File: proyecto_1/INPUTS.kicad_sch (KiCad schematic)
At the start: 0 parts

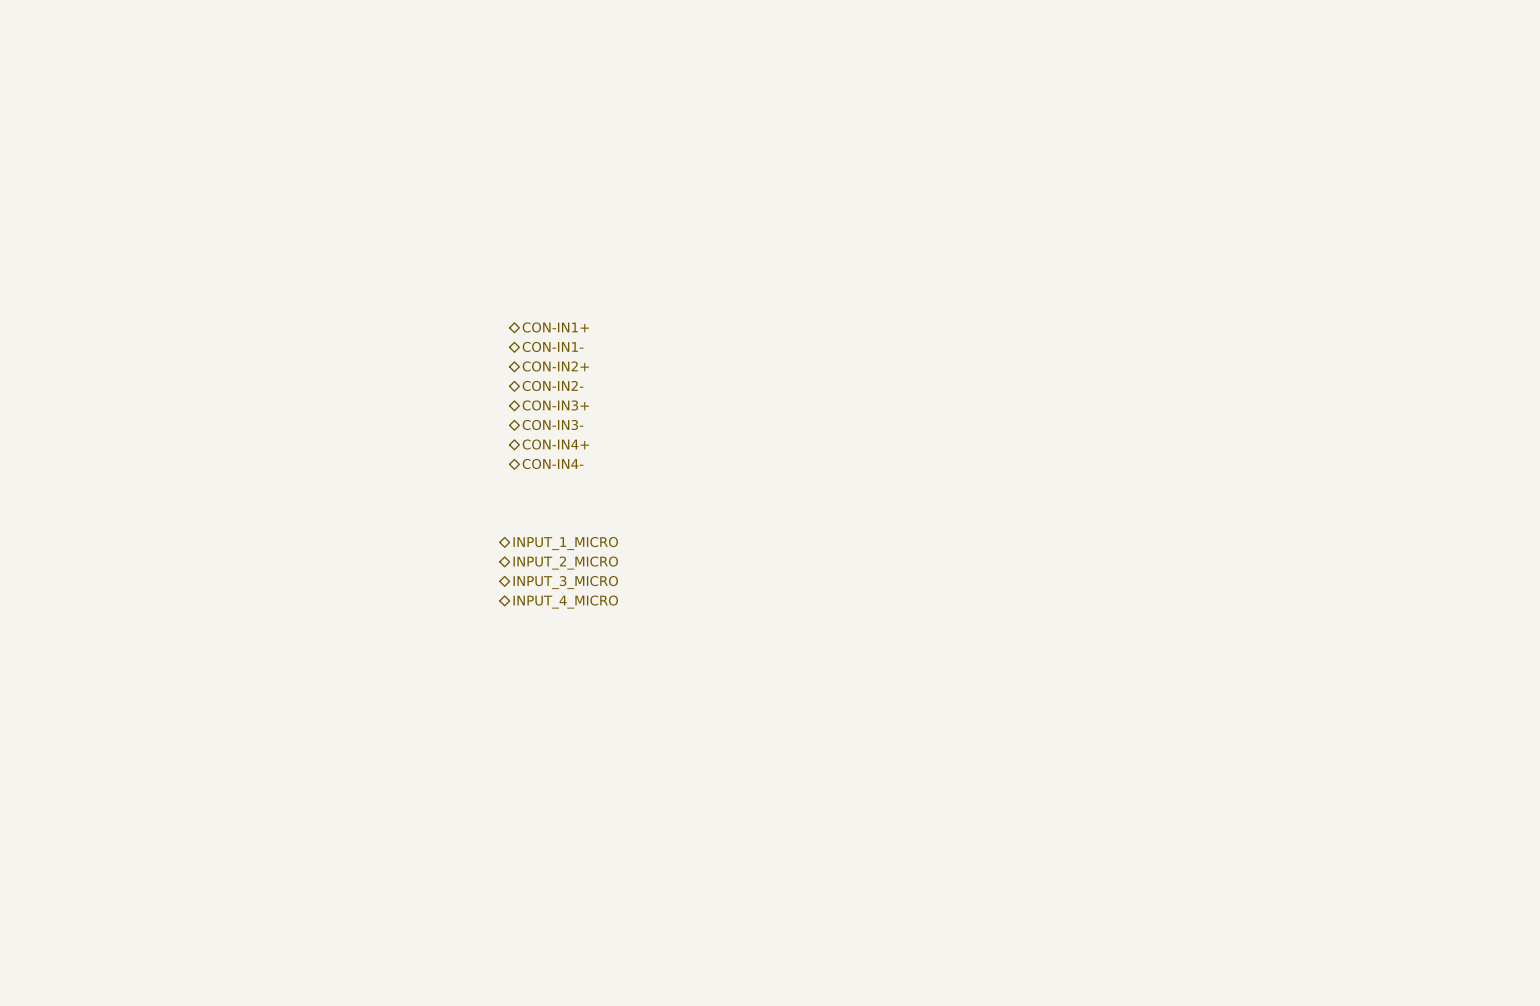
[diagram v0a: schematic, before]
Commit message: nuevos circuitos de pcb
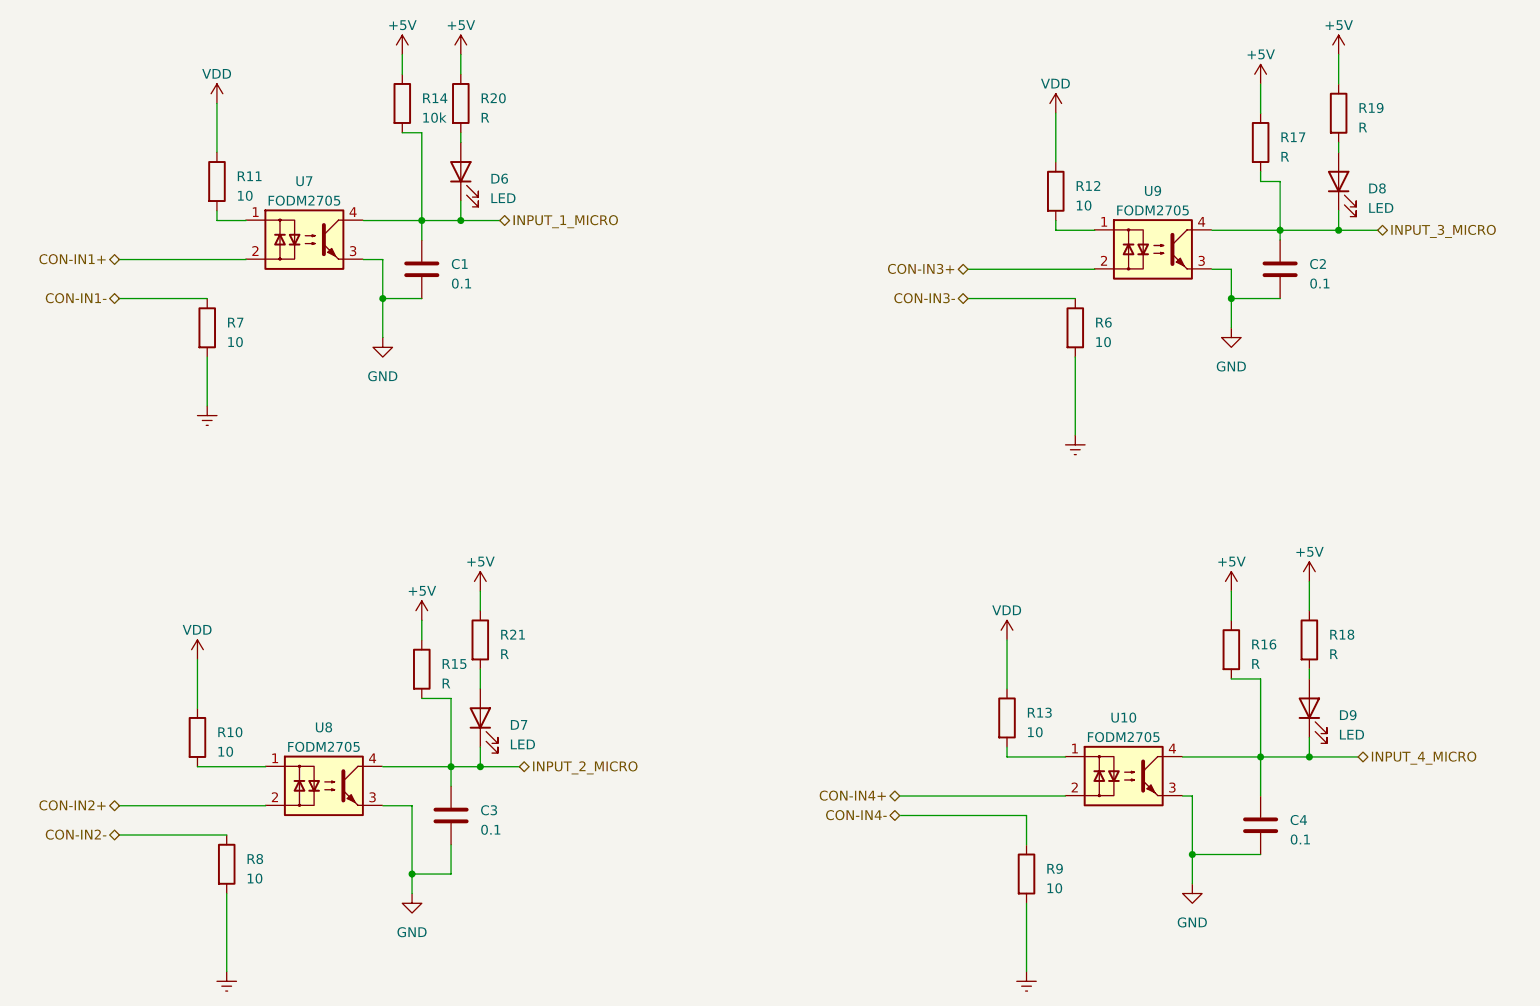
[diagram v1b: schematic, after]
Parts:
- added C1, C2, C3, C4: 0.1, symbol Device:C
- added D6, D7, D8, D9: LED, symbol Device:LED
- added R10, R11, R12, R13, R6, R7, R8, R9: 10, symbol Device:R
- added R14: 10k, symbol Device:R
- added R15, R16, R17, R18, R19, R20, R21: R, symbol Device:R
- added U10, U7, U8, U9: FODM2705, nuevo simbolo:FODM2705, symbol nuevo simbolos:FODM2705
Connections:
- net CON-IN1-: now also R7.1
- net CON-IN2-: now also R8.1
- net CON-IN3-: now also R6.1
- net CON-IN4-: now also R9.1
- net INPUT_1_MICRO: now also C1.1, D6.1 (K), R14.2
- net INPUT_2_MICRO: now also C3.1, D7.1 (K), R15.2
- net INPUT_3_MICRO: now also C2.1, D8.1 (K), R17.2
- net INPUT_4_MICRO: now also C4.1, D9.1 (K), R16.2
- new net: D8.2 (A), R19.2
- new net: D9.2 (A), R18.2
- new net: D6.2 (A), R20.2
- new net: D7.2 (A), R21.2
- new net +5V: R14.1, R15.1, R16.1, R17.1, R18.1, R19.1, R20.1, R21.1
- new net Earth: R6.2, R7.2, R8.2, R9.2
- new net GND: C1.2, C2.2, C3.2, C4.2
- new net VDD: R10.1, R11.1, R12.1, R13.1

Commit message: agregados al esquematico
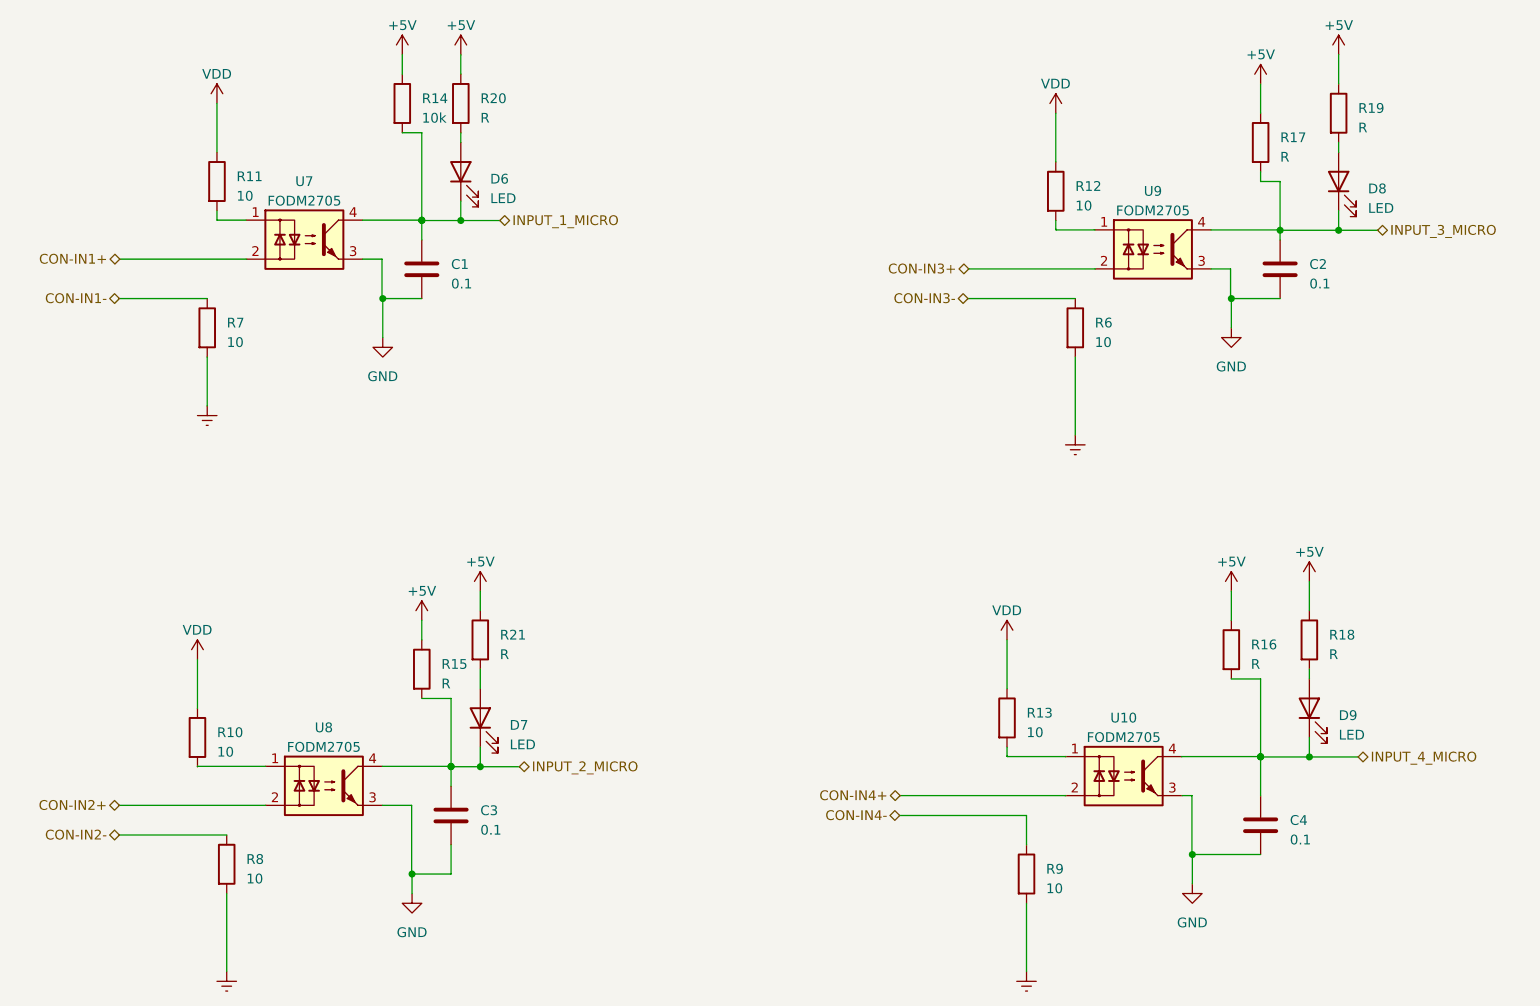
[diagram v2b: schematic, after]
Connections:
- net GND: now also U10.3, U8.3
- net INPUT_2_MICRO: now also U8.4
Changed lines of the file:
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@@
   (junction (at 214.63 64.77) (diameter 0) (color 0 0 0 0)
   )
+  (junction (at 99.06 134.5692) (diameter 0) (color 0 0 0 0)
+  )
   (junction (at 102.87 134.62) (diameter 0) (color 0 0 0 0)
   )
@@
   (junction (at 100.33 63.5) (diameter 0) (color 0 0 0 0)
   )
+  (junction (at 204.47 133.2992) (diameter 0) (color 0 0 0 0)
+  )
   (junction (at 95.25 63.5) (diameter 0) (color 0 0 0 0)
   )
@@
   (junction (at 99.06 134.62) (diameter 0) (color 0 0 0 0)
   )
+  (junction (at 95.25 63.4492) (diameter 0) (color 0 0 0 0)
+  )
   (junction (at 207.01 64.77) (diameter 0) (color 0 0 0 0)
   )
-  (wire (pts (xy 177.8 64.77) (xy 177.8 63.5))
+  (wire (pts (xy 171.45 133.2484) (xy 171.45 132.08))
+    (stroke (width 0) (type default))
+  )
+  (wire (pts (xy 177.8508 64.7192) (xy 177.8508 64.6684))
     (stroke (width 0) (type default))
   )
@@
     (stroke (width 0) (type default))
   )
+  (wire (pts (xy 90.1192 134.5692) (xy 99.06 134.5692))
+    (stroke (width 0) (type default))
+  )
   (wire (pts (xy 100.33 60.96) (xy 100.33 63.5))
     (stroke (width 0) (type default))
@@
     (stroke (width 0) (type default))
   )
-  (wire (pts (xy 179.07 133.35) (xy 171.45 133.35))
+  (wire (pts (xy 195.5292 146.05) (xy 195.58 146.05))
+    (stroke (width 0) (type default))
+  )
+  (wire (pts (xy 66.04 134.5692) (xy 66.04 134.62))
+    (stroke (width 0) (type default))
+  )
+  (wire (pts (xy 177.8 64.6684) (xy 177.8 63.5))
     (stroke (width 0) (type default))
   )
@@
     (stroke (width 0) (type default))
   )
+  (wire (pts (xy 206.9084 64.77) (xy 207.01 64.77))
+    (stroke (width 0) (type default))
+  )
+  (wire (pts (xy 90.0684 73.66) (xy 90.17 73.66))
+    (stroke (width 0) (type default))
+  )
   (wire (pts (xy 95.25 125.73) (xy 99.06 125.73))
     (stroke (width 0) (type default))
   )
-  (wire (pts (xy 72.39 63.5) (xy 68.58 63.5))
+  (wire (pts (xy 68.58 63.4492) (xy 72.39 63.4492))
     (stroke (width 0) (type default))
   )
@@
     (stroke (width 0) (type default))
   )
-  (wire (pts (xy 200.66 69.85) (xy 200.66 73.66))
+  (wire (pts (xy 200.5584 69.7992) (xy 200.5584 73.66))
     (stroke (width 0) (type default))
   )
@@
     (stroke (width 0) (type default))
   )
+  (wire (pts (xy 198.0184 69.7992) (xy 200.5584 69.7992))
+    (stroke (width 0) (type default))
+  )
   (wire (pts (xy 210.82 130.81) (xy 210.82 133.35))
     (stroke (width 0) (type default))
@@
     (stroke (width 0) (type default))
   )
+  (wire (pts (xy 99.06 134.5692) (xy 99.06 134.62))
+    (stroke (width 0) (type default))
+  )
   (wire (pts (xy 69.85 151.13) (xy 69.85 161.29))
     (stroke (width 0) (type default))
@@
     (stroke (width 0) (type default))
   )
+  (wire (pts (xy 204.47 133.2992) (xy 204.47 133.35))
+    (stroke (width 0) (type default))
+  )
   (wire (pts (xy 55.88 143.51) (xy 69.85 143.51))
     (stroke (width 0) (type default))
@@
     (stroke (width 0) (type default))
   )
-  (wire (pts (xy 194.31 133.35) (xy 204.47 133.35))
-    (stroke (width 0) (type default))
-  )
-  (wire (pts (xy 55.88 68.58) (xy 72.39 68.58))
-    (stroke (width 0) (type default))
-  )
-  (wire (pts (xy 93.98 139.7) (xy 93.98 148.59))
-    (stroke (width 0) (type default))
-  )
-  (wire (pts (xy 204.47 123.19) (xy 204.47 133.35))
-    (stroke (width 0) (type default))
-  )
-  (wire (pts (xy 66.04 134.62) (xy 74.93 134.62))
+  (wire (pts (xy 194.1576 133.2992) (xy 204.47 133.2992))
+    (stroke (width 0) (type default))
+  )
+  (wire (pts (xy 93.9292 139.6492) (xy 93.9292 148.59))
+    (stroke (width 0) (type default))
+  )
+  (wire (pts (xy 204.47 123.19) (xy 204.47 133.2992))
+    (stroke (width 0) (type default))
+  )
+  (wire (pts (xy 66.04 134.5692) (xy 74.93 134.5692))
     (stroke (width 0) (type default))
   )
@@
     (stroke (width 0) (type default))
   )
-  (wire (pts (xy 87.63 63.5) (xy 95.25 63.5))
-    (stroke (width 0) (type default))
-  )
-  (wire (pts (xy 194.31 138.43) (xy 195.58 138.43))
+  (wire (pts (xy 171.5008 133.2992) (xy 179.1208 133.2992))
+    (stroke (width 0) (type default))
+  )
+  (wire (pts (xy 95.25 63.4492) (xy 95.25 63.5))
+    (stroke (width 0) (type default))
+  )
+  (wire (pts (xy 194.2592 138.3792) (xy 195.5292 138.3792))
     (stroke (width 0) (type default))
   )
@@
     (stroke (width 0) (type default))
   )
-  (wire (pts (xy 95.25 52.07) (xy 95.25 63.5))
+  (wire (pts (xy 95.25 52.07) (xy 95.25 63.4492))
     (stroke (width 0) (type default))
   )
@@
     (stroke (width 0) (type default))
   )
-  (wire (pts (xy 166.37 69.85) (xy 182.88 69.85))
-    (stroke (width 0) (type default))
-  )
   (wire (pts (xy 195.58 146.05) (xy 204.47 146.05))
     (stroke (width 0) (type default))
   )
+  (wire (pts (xy 93.9292 148.59) (xy 93.98 148.59))
+    (stroke (width 0) (type default))
+  )
+  (wire (pts (xy 87.5284 63.4492) (xy 95.25 63.4492))
+    (stroke (width 0) (type default))
+  )
   (wire (pts (xy 204.47 45.72) (xy 204.47 49.53))
     (stroke (width 0) (type default))
   )
-  (wire (pts (xy 198.12 69.85) (xy 200.66 69.85))
-    (stroke (width 0) (type default))
-  )
-  (wire (pts (xy 157.48 138.43) (xy 179.07 138.43))
-    (stroke (width 0) (type default))
-  )
   (wire (pts (xy 214.63 53.34) (xy 214.63 54.61))
     (stroke (width 0) (type default))
   )
-  (wire (pts (xy 87.63 68.58) (xy 90.17 68.58))
+  (wire (pts (xy 200.5584 73.66) (xy 200.66 73.66))
+    (stroke (width 0) (type default))
+  )
+  (wire (pts (xy 55.9308 68.5292) (xy 72.4408 68.5292))
     (stroke (width 0) (type default))
   )
@@
     (stroke (width 0) (type default))
   )
-  (wire (pts (xy 195.58 138.43) (xy 195.58 146.05))
+  (wire (pts (xy 198.0184 64.7192) (xy 206.9084 64.7192))
+    (stroke (width 0) (type default))
+  )
+  (wire (pts (xy 177.8508 64.7192) (xy 182.9308 64.7192))
+    (stroke (width 0) (type default))
+  )
+  (wire (pts (xy 195.5292 138.3792) (xy 195.5292 146.05))
+    (stroke (width 0) (type default))
+  )
+  (wire (pts (xy 166.4716 69.7992) (xy 182.9816 69.7992))
     (stroke (width 0) (type default))
   )
@@
     (stroke (width 0) (type default))
   )
+  (wire (pts (xy 177.8508 64.6684) (xy 177.8 64.6684))
+    (stroke (width 0) (type default))
+  )
   (wire (pts (xy 204.47 58.42) (xy 207.01 58.42))
     (stroke (width 0) (type default))
   )
-  (wire (pts (xy 55.88 139.7) (xy 74.93 139.7))
+  (wire (pts (xy 55.88 139.6492) (xy 74.93 139.6492))
     (stroke (width 0) (type default))
   )
@@
     (stroke (width 0) (type default))
   )
-  (wire (pts (xy 68.58 63.5) (xy 68.58 62.23))
+  (wire (pts (xy 68.58 63.4492) (xy 68.58 62.23))
     (stroke (width 0) (type default))
   )
@@
     (stroke (width 0) (type default))
   )
-  (wire (pts (xy 90.17 134.62) (xy 99.06 134.62))
-    (stroke (width 0) (type default))
-  )
   (wire (pts (xy 92.71 52.07) (xy 95.25 52.07))
     (stroke (width 0) (type default))
   )
-  (wire (pts (xy 90.17 68.58) (xy 90.17 73.66))
-    (stroke (width 0) (type default))
-  )
-  (wire (pts (xy 182.88 64.77) (xy 177.8 64.77))
-    (stroke (width 0) (type default))
-  )
-  (wire (pts (xy 171.45 133.35) (xy 171.45 132.08))
+  (wire (pts (xy 90.0684 68.5292) (xy 90.0684 73.66))
+    (stroke (width 0) (type default))
+  )
+  (wire (pts (xy 171.5008 133.2992) (xy 171.5008 133.2484))
     (stroke (width 0) (type default))
   )
@@
     (stroke (width 0) (type default))
   )
-  (wire (pts (xy 99.06 125.73) (xy 99.06 134.62))
+  (wire (pts (xy 99.06 125.73) (xy 99.06 134.5692))
     (stroke (width 0) (type default))
   )
@@
     (stroke (width 0) (type default))
   )
-  (wire (pts (xy 90.17 139.7) (xy 93.98 139.7))
+  (wire (pts (xy 157.5308 138.3792) (xy 179.1208 138.3792))
+    (stroke (width 0) (type default))
+  )
+  (wire (pts (xy 90.1192 139.6492) (xy 93.9292 139.6492))
+    (stroke (width 0) (type default))
+  )
+  (wire (pts (xy 87.5284 68.5292) (xy 90.0684 68.5292))
     (stroke (width 0) (type default))
   )
@@
     (stroke (width 0) (type default))
   )
-  (wire (pts (xy 198.12 64.77) (xy 207.01 64.77))
-    (stroke (width 0) (type default))
-  )
-  (hierarchical_label "CON-IN1+" (shape bidirectional) (at 55.88 68.58 180) (fields_autoplaced)
+  (wire (pts (xy 171.5008 133.2484) (xy 171.45 133.2484))
+    (stroke (width 0) (type default))
+  )
+  (wire (pts (xy 206.9084 64.7192) (xy 206.9084 64.77))
+    (stroke (width 0) (type default))
+  )
+  (hierarchical_label "CON-IN1+" (shape bidirectional) (at 55.9308 68.5292 180) (fields_autoplaced)
     (effects (font (size 1.27 1.27)) (justify right))
   )
@@
     (effects (font (size 1.27 1.27)) (justify left))
   )
-  (hierarchical_label "CON-IN4+" (shape bidirectional) (at 157.48 138.43 180) (fields_autoplaced)
+  (hierarchical_label "CON-IN4+" (shape bidirectional) (at 157.5308 138.3792 180) (fields_autoplaced)
     (effects (font (size 1.27 1.27)) (justify right))
   )
@@
     (effects (font (size 1.27 1.27)) (justify right))
   )
-  (hierarchical_label "CON-IN2+" (shape bidirectional) (at 55.88 139.7 180) (fields_autoplaced)
+  (hierarchical_label "CON-IN2+" (shape bidirectional) (at 55.88 139.6492 180) (fields_autoplaced)
     (effects (font (size 1.27 1.27)) (justify right))
   )
@@
     (effects (font (size 1.27 1.27)) (justify right))
   )
-  (hierarchical_label "CON-IN3+" (shape bidirectional) (at 166.37 69.85 180) (fields_autoplaced)
-    (effects (font (size 1.27 1.27)) (justify right))
-  )
+  (hierarchical_label "CON-IN3+" (shape bidirectional) (at 166.4716 69.7992 180) (fields_autoplaced)
+    (effects (font (size 1.27 1.27)) (justify right))
+  )
